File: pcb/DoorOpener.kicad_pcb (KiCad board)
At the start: 2 copper layers, 50.8 x 37.8 mm, 7 parts, among them SW1 POWER, SW2 Button, U2 ESP-01v090

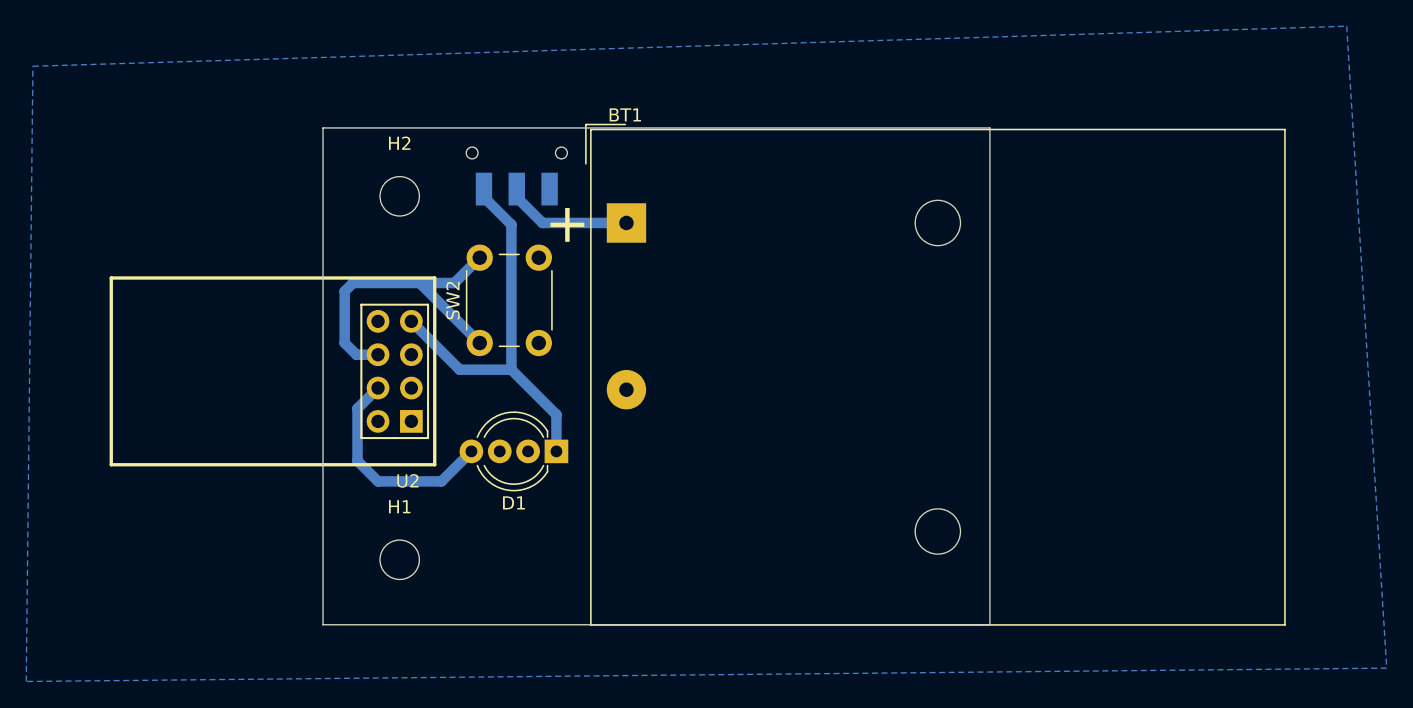
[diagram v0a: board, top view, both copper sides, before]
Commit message: Prepare for milling the pcb
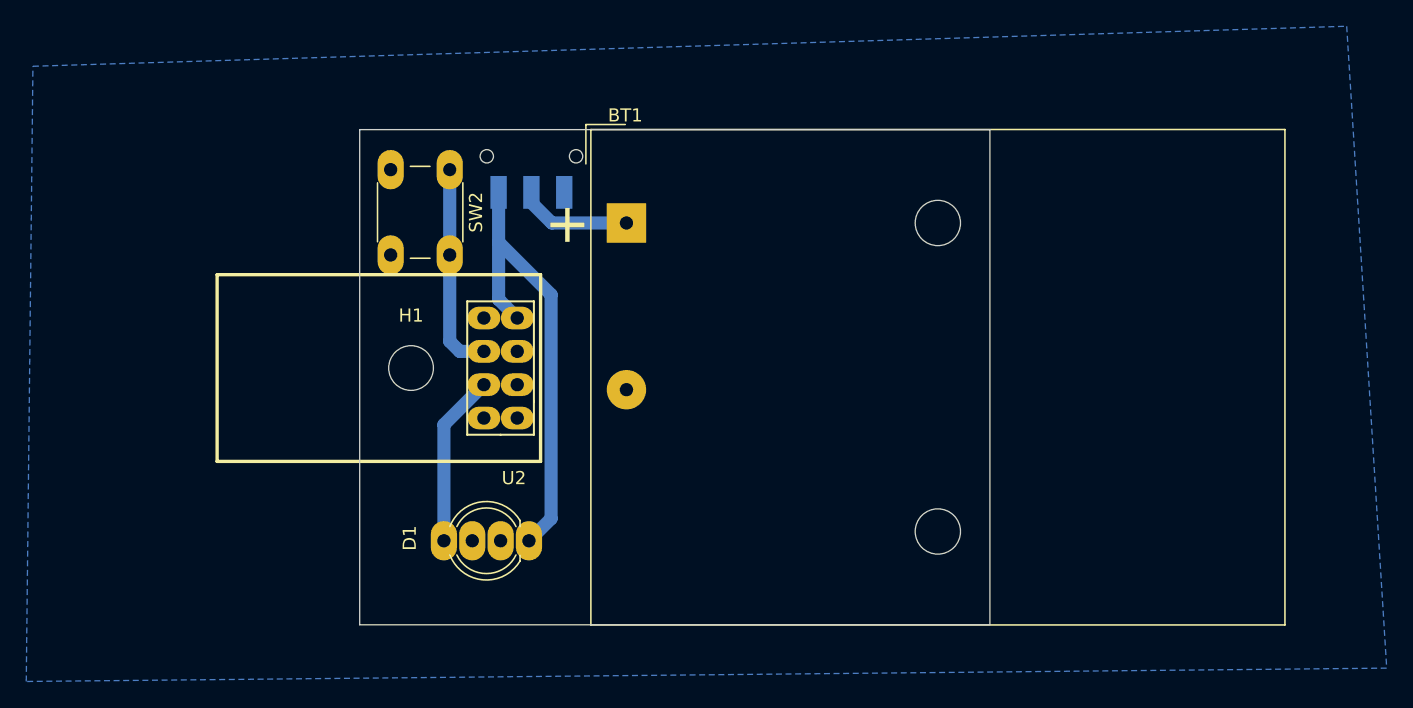
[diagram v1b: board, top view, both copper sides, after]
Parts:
- removed H2: MountingHole, MountingHole:MountingHole_3mm
- moved H1 14.6 mm to (76.0, 140.7)
- moved SW2 13.4 mm to (79.0, 125.6), turned to -90 degrees
- moved U2 8.07 mm to (84.1, 144.5)
- moved D1 7.12 mm to (85.0, 153.9)
- moved SW1 1.14 mm to (85.2, 124.6)
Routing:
- net Net-(SW2-Pad1): track 24.7 -> 16.0 mm
- net +3V3: track 31.5 -> 35.0 mm
- net Net-(D1-Pad4): track 16.5 -> 13.1 mm
- net Net-(BT1-Pad1): track 9.79 -> 8.40 mm
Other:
- board size 50.8 x 37.8 mm -> 48 x 37.7 mm
- board text added: "v0.1 - 17.11.2022"
